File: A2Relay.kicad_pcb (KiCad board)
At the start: 2 copper layers, 33 x 30.5 mm, 8 parts, among them J1 Gameport, J2 Gamepad, J3 /RESET, J4 RELAY, U1 SN74ALS259, U2 SN74ALS259DR

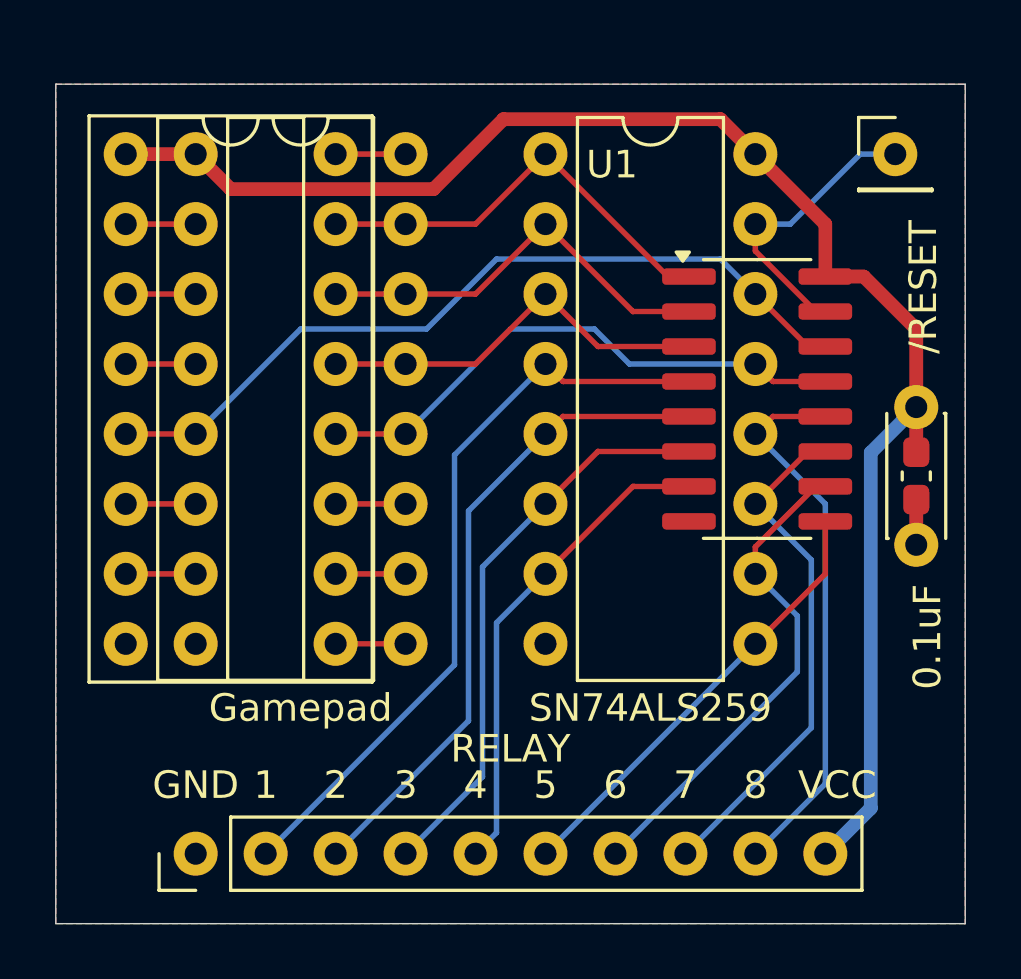
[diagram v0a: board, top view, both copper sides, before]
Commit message: revision 3 - initial prototype run
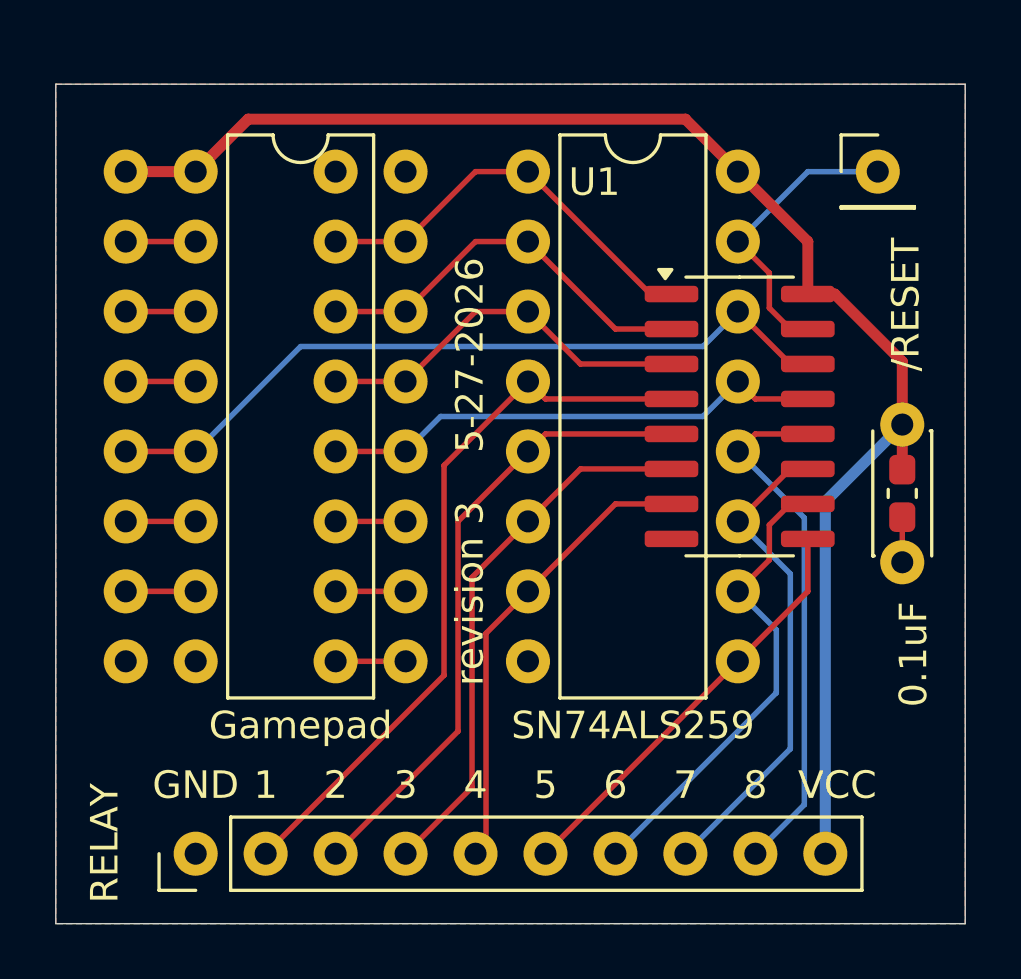
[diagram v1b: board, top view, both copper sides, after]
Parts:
- added G***: LOGO, cityxen:deadline97, B.Cu at (102.0, 56.8)
- moved J3 0.90 mm to (111.1, 46.4)
- moved U1 0.90 mm to (98.4, 46.4)
- moved U2 0.90 mm to (106.1, 55.2)
- moved C1 0.81 mm to (112.0, 55.5)
- moved C2 0.81 mm to (112.0, 58.0)
- moved J1 0.63 mm to (83.8, 46.4)
- moved J2 0.63 mm to (86.4, 46.4)
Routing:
- net RESERVED: track 2.54 -> 0.00 mm
- net +5V: track 56.6 -> 54.4 mm
- net AN3: track 20.1 -> 18.5 mm
- net /STB: track 29.3 -> 27.7 mm
- net Q7: track 20.1 -> 19.1 mm
- net Q6: track 18.8 -> 17.8 mm
- net Q4: track 16.3 -> 15.4 mm
- net Q1: track 23.9 -> 23.0 mm
- net Q3: track 17.7 -> 16.8 mm
- net Q0: track 27.5 -> 26.6 mm
- net Q2: track 20.8 -> 19.9 mm
- net Q5: track 18.0 -> 17.1 mm
- net AN2: track 14.7 -> 14.0 mm
- net AN1: track 15.2 -> 14.6 mm
- net AN0: track 15.7 -> 15.1 mm
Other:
- board text added: "&"
- board text added: "Apple II Relay Board"
- board text added: "CityXen"
- board text added: "V2"
- board text added: "V2 Retro Computing"
- board text added: "by"
- board text added: "designed for"
- board text added: "revision 3 5-27-2026"
- board text added: "© 2026 David Kuder"
